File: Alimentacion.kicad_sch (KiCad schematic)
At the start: 5 parts, among them J1 1366004

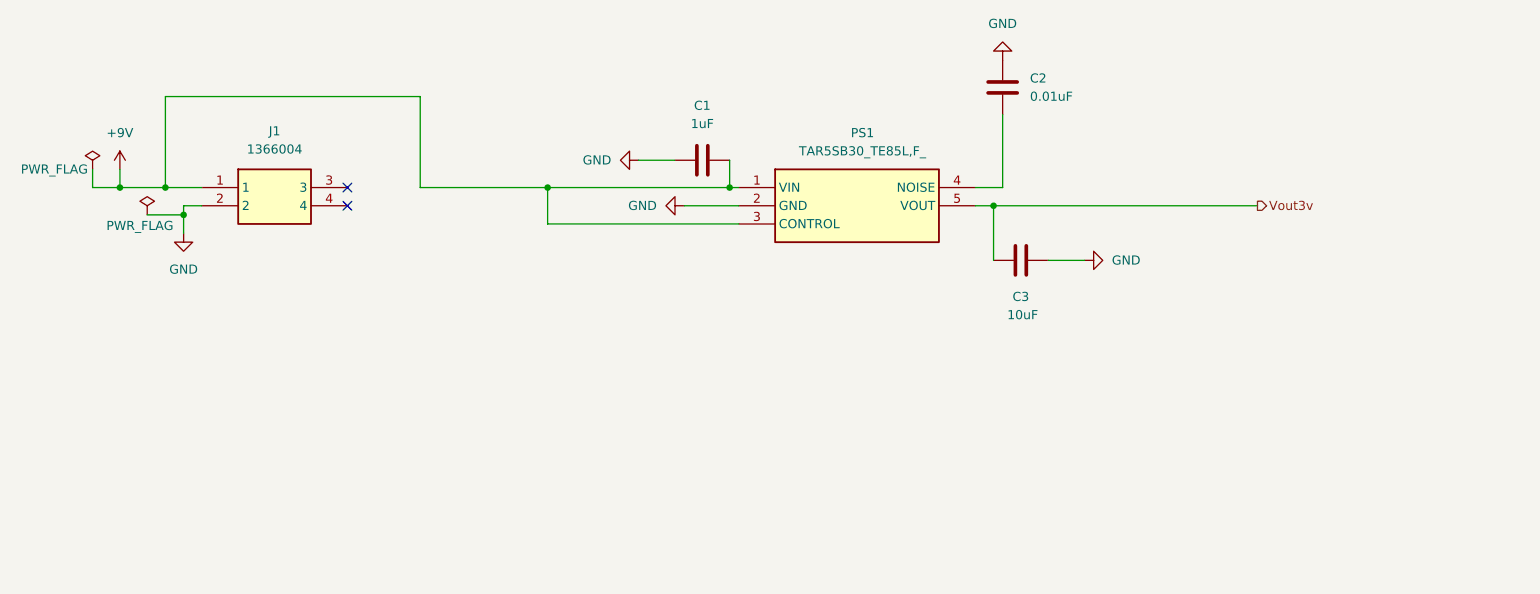
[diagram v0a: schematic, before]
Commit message: sesion 4
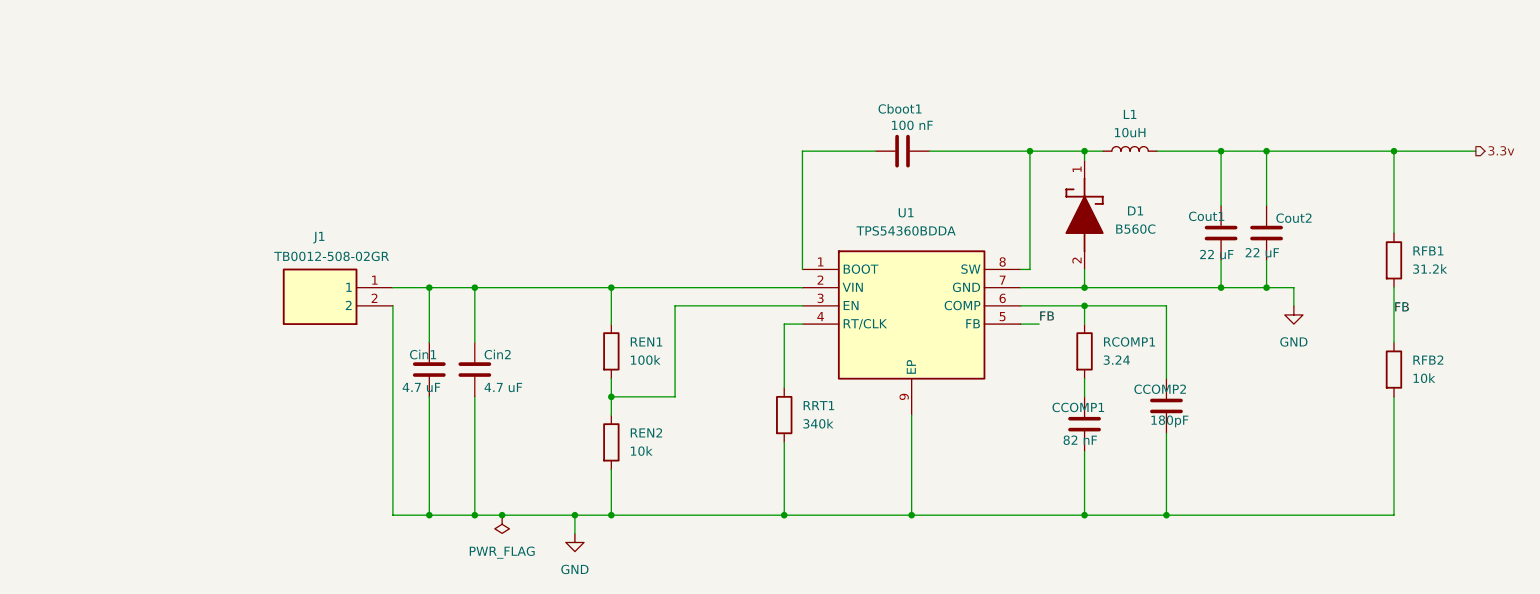
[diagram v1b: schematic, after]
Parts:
- removed C1: 1uF, Capacitor_SMD:C_0402_1005Metric, symbol Device:C
- removed C2: 0.01uF, Capacitor_SMD:C_0402_1005Metric, symbol Device:C
- removed C3: 10uF, Capacitor_SMD:C_0402_1005Metric, symbol Device:C
- removed J1: 1366004, Samacsys:1366004, symbol Samacsys:1366004
- removed PS1: TAR5SB30_TE85L,F_, Samacsys:SOT95P275X140-5N, symbol Samacsys:TAR5SB30_TE85L,F_
- added CCOMP1: 82 nF, Capacitor_SMD:C_0402_1005Metric, symbol Device:C
- added CCOMP2: 180pF, Capacitor_SMD:C_0402_1005Metric, symbol Device:C
- added Cboot1: 100 nF, Capacitor_SMD:C_0402_1005Metric, symbol Device:C
- added Cin1, Cin2: 4.7 uF, Capacitor_SMD:C_0402_1005Metric, symbol Device:C
- added Cout1, Cout2: 22 uF, Capacitor_SMD:C_0402_1005Metric, symbol Device:C
- added D1: B560C, Samacsys:DIOM7959X250N, symbol Samacsys:B560C
- added J1: TB0012-508-02GR, Samacsys:TB0012-508-02GR, symbol Samacsys:TB0012-508-02GR
- added L1: 10uH, Inductor_SMD:L_1206_3216Metric, symbol Device:L
- added RCOMP1: 3.24, Resistor_SMD:R_0402_1005Metric_Pad0.72x0.64mm_HandSolder, symbol Device:R
- added REN1: 100k, Resistor_SMD:R_0402_1005Metric_Pad0.72x0.64mm_HandSolder, symbol Device:R
- added REN2, RFB2: 10k, Resistor_SMD:R_0402_1005Metric_Pad0.72x0.64mm_HandSolder, symbol Device:R
- added RFB1: 31.2k, Resistor_SMD:R_0402_1005Metric_Pad0.72x0.64mm_HandSolder, symbol Device:R
- added RRT1: 340k, Resistor_SMD:R_0402_1005Metric_Pad0.72x0.64mm_HandSolder, symbol Device:R
- added U1: TPS54360BDDA, Samacsys:SOIC127P600X170-9N, symbol Samacsys:TPS54360BDDA
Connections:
- net GND: now also CCOMP1.2, CCOMP2.2, Cin1.2, Cin2.2, Cout1.2, Cout2.2, D1.2 (A), J1.2, REN2.2, RFB2.2, RRT1.2, U1.7 (GND), U1.9 (EP)
- new net: CCOMP2.1, RCOMP1.1, U1.6 (COMP)
- new net: RRT1.1, U1.4 (RT/CLK)
- new net: Cboot1.1, U1.1 (BOOT)
- new net: Cin1.1, Cin2.1, J1.1, REN1.1, U1.2 (VIN)
- new net: REN1.2, REN2.1, U1.3 (EN)
- new net: Cboot1.2, D1.1 (K), L1.1, U1.8 (SW)
- new net: CCOMP1.1, RCOMP1.2
- new net 3.3v: Cout1.1, Cout2.1, L1.2, RFB1.1
- new net FB: RFB1.2, RFB2.1, U1.5 (FB)
- no-connect marks 2 -> 0
